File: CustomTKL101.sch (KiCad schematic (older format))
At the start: 220 parts, among them J1 USB4085-GF-A_REVA, SW1 SW_Push, U1 ATmega32U4-AU, Y1 16MHz

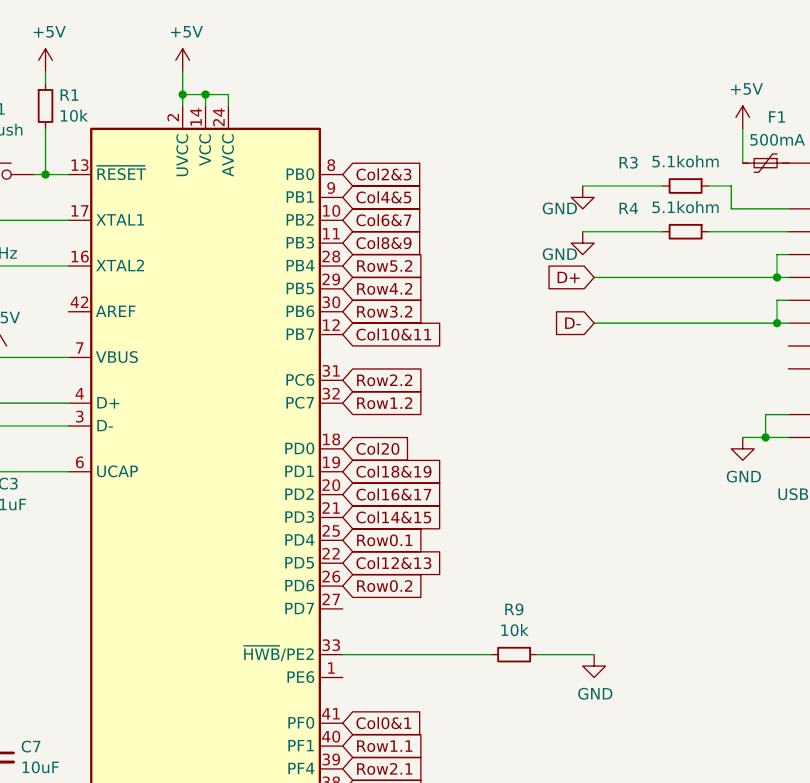
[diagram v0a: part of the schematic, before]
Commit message: Completed PCB ?
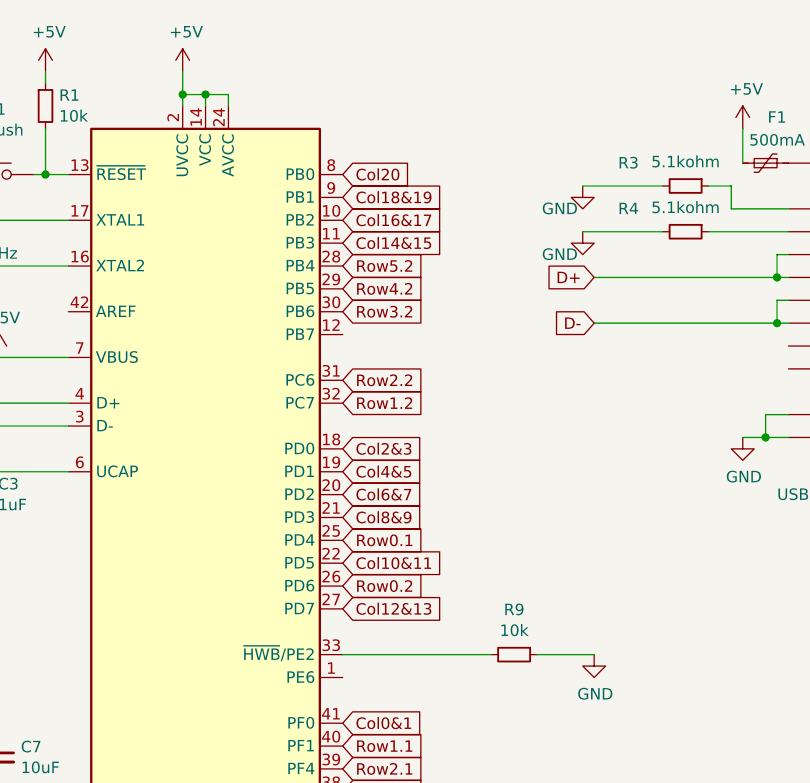
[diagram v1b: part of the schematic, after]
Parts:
- MX101, MX32: footprint MX_Alps_Hybrid:MX-1U-NoLED -> MX_Alps_Hybrid:MX-2U-ReversedStabilizers-NoLED
- MX71, MX75: footprint MX_Alps_Hybrid:MX-1U-NoLED -> MX_Alps_Hybrid:MX-2.25U-ReversedStabilizers-NoLED
- MX86: footprint MX_Alps_Hybrid:MX-1U-NoLED -> MX_Alps_Hybrid:MX-2.75U-ReversedStabilizers-NoLED
- MX93: footprint MX_Alps_Hybrid:MX-1U-NoLED -> MX_Alps_Hybrid:MX-6.25U-ReversedStabilizers-NoLED
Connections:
- net Col10&11: now also U1.22 (PD5); no longer U1.12 (PB7)
- net Col12&13: now also U1.27 (PD7); no longer U1.22 (PD5)
- net Col14&15: now also U1.11 (PB3); no longer U1.21 (PD3)
- net Col16&17: now also U1.10 (PB2); no longer U1.20 (PD2)
- net Col18&19: now also U1.9 (PB1); no longer U1.19 (PD1)
- net Col2&3: now also U1.18 (PD0); no longer U1.8 (PB0)
- net Col20: now also U1.8 (PB0); no longer U1.18 (PD0)
- net Col4&5: now also U1.19 (PD1); no longer U1.9 (PB1)
- net Col6&7: now also U1.20 (PD2); no longer U1.10 (PB2)
- net Col8&9: now also U1.21 (PD3); no longer U1.11 (PB3)
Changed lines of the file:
@@
 F 0 "MX93" H 7783 5723 60  0000 C CNN
 F 1 "MX-NoLED" H 7783 5649 20  0000 C CNN
-F 2 "MX_Alps_Hybrid:MX-1U-NoLED" H 7125 5475 60  0001 C CNN
+F 2 "MX_Alps_Hybrid:MX-6.25U-ReversedStabilizers-NoLED" H 7125 5475 60  0001 C CNN
 F 3 "" H 7125 5475 60  0001 C CNN
 	1    7750 5500
@@
 F 0 "MX86" H 11683 4973 60  0000 C CNN
 F 1 "MX-NoLED" H 11683 4899 20  0000 C CNN
-F 2 "MX_Alps_Hybrid:MX-1U-NoLED" H 11025 4725 60  0001 C CNN
+F 2 "MX_Alps_Hybrid:MX-2.75U-ReversedStabilizers-NoLED" H 11025 4725 60  0001 C CNN
 F 3 "" H 11025 4725 60  0001 C CNN
 	1    11650 4750
@@
 F 0 "MX71" H 12333 4223 60  0000 C CNN
 F 1 "MX-NoLED" H 12333 4149 20  0000 C CNN
-F 2 "MX_Alps_Hybrid:MX-1U-NoLED" H 11675 3975 60  0001 C CNN
+F 2 "MX_Alps_Hybrid:MX-2.25U-ReversedStabilizers-NoLED" H 11675 3975 60  0001 C CNN
 F 3 "" H 11675 3975 60  0001 C CNN
 	1    12300 4000
@@
 F 0 "MX32" H 12333 2723 60  0000 C CNN
 F 1 "MX-NoLED" H 12333 2649 20  0000 C CNN
-F 2 "MX_Alps_Hybrid:MX-1U-NoLED" H 11675 2475 60  0001 C CNN
+F 2 "MX_Alps_Hybrid:MX-2U-ReversedStabilizers-NoLED" H 11675 2475 60  0001 C CNN
 F 3 "" H 11675 2475 60  0001 C CNN
 	1    12300 2500
@@
 F 0 "MX101" H 14933 5723 60  0000 C CNN
 F 1 "MX-NoLED" H 14933 5649 20  0000 C CNN
-F 2 "MX_Alps_Hybrid:MX-1U-NoLED" H 14275 5475 60  0001 C CNN
+F 2 "MX_Alps_Hybrid:MX-2U-ReversedStabilizers-NoLED" H 14275 5475 60  0001 C CNN
 F 3 "" H 14275 5475 60  0001 C CNN
 	1    14900 5500
@@
 F 0 "MX75" H 3883 4973 60  0000 C CNN
 F 1 "MX-NoLED" H 3883 4899 20  0000 C CNN
-F 2 "MX_Alps_Hybrid:MX-1U-NoLED" H 3225 4725 60  0001 C CNN
+F 2 "MX_Alps_Hybrid:MX-2.25U-ReversedStabilizers-NoLED" H 3225 4725 60  0001 C CNN
 F 3 "" H 3225 4725 60  0001 C CNN
 	1    3850 4750
@@
 Text GLabel 3400 9950 2    50   Input ~ 0
 Col0&1
-Text GLabel 3400 8750 2    50   Input ~ 0
-Col20
-Text GLabel 3400 8850 2    50   Input ~ 0
-Col18&19
-Text GLabel 3400 8950 2    50   Input ~ 0
-Col16&17
-Text GLabel 3400 9050 2    50   Input ~ 0
-Col14&15
-Text GLabel 3400 9250 2    50   Input ~ 0
-Col12&13
-Text GLabel 3400 8250 2    50   Input ~ 0
-Col10&11
-Text GLabel 3400 7850 2    50   Input ~ 0
-Col8&9
-Text GLabel 3400 7750 2    50   Input ~ 0
-Col6&7
-Text GLabel 3400 7650 2    50   Input ~ 0
-Col4&5
-Text GLabel 3400 7550 2    50   Input ~ 0
-Col2&3
 Text GLabel 3400 9150 2    50   Input ~ 0
 Row0.1
@@
 Wire Wire Line
 	4500 8200 5300 8200
+Text GLabel 3400 7550 2    50   Input ~ 0
+Col20
+Text GLabel 3400 7650 2    50   Input ~ 0
+Col18&19
+Text GLabel 3400 7750 2    50   Input ~ 0
+Col16&17
+Text GLabel 3400 7850 2    50   Input ~ 0
+Col14&15
+Text GLabel 3400 9450 2    50   Input ~ 0
+Col12&13
+Text GLabel 3400 9250 2    50   Input ~ 0
+Col10&11
+Text GLabel 3400 9050 2    50   Input ~ 0
+Col8&9
+Text GLabel 3400 8950 2    50   Input ~ 0
+Col6&7
+Text GLabel 3400 8850 2    50   Input ~ 0
+Col4&5
+Text GLabel 3400 8750 2    50   Input ~ 0
+Col2&3
 $EndSCHEMATC
